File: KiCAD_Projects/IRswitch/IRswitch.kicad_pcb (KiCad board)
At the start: 2 copper layers, 39.4 x 45.7 mm, 14 parts, among them IC1 ATMEGA168-P, P1 CONN_01X02, P2 CONN_01X03, P3 CONN_01X05, Q1 MOSFET_N, X1 CRYSTAL

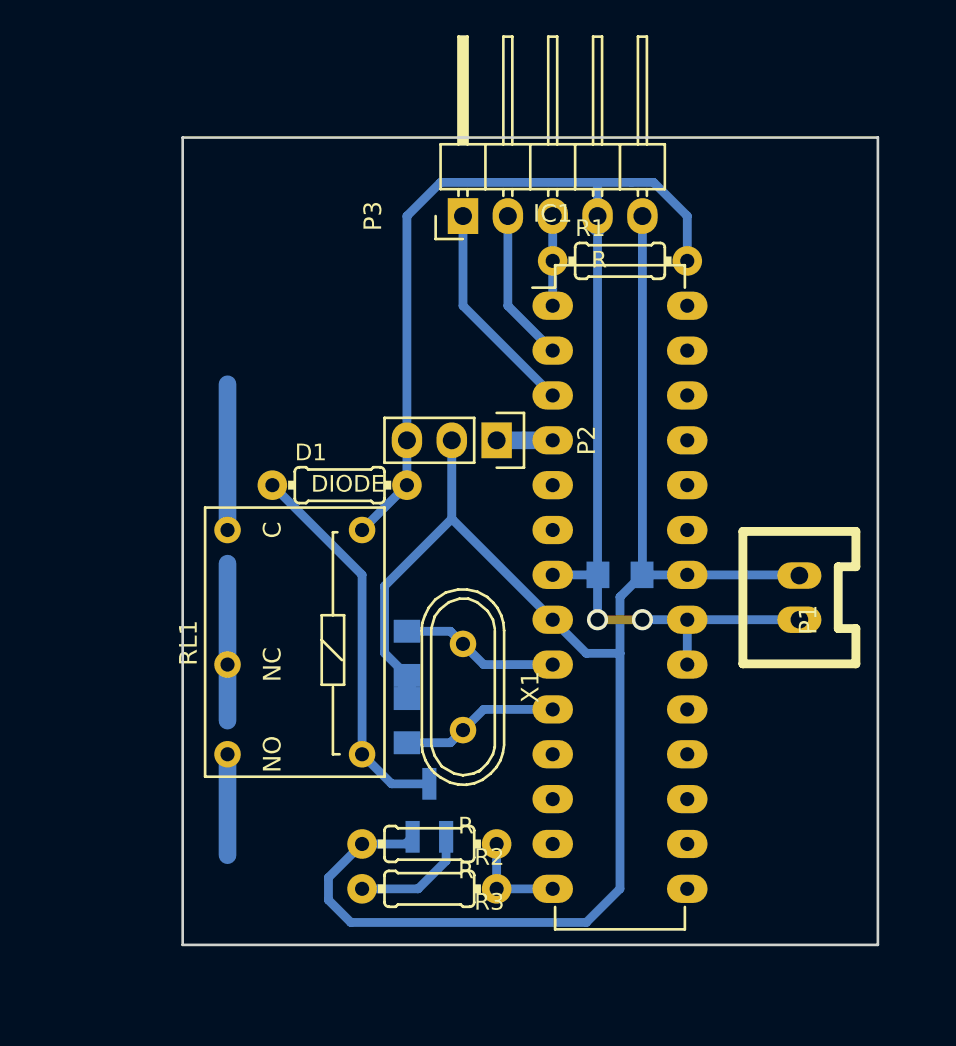
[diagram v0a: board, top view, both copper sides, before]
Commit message: no message
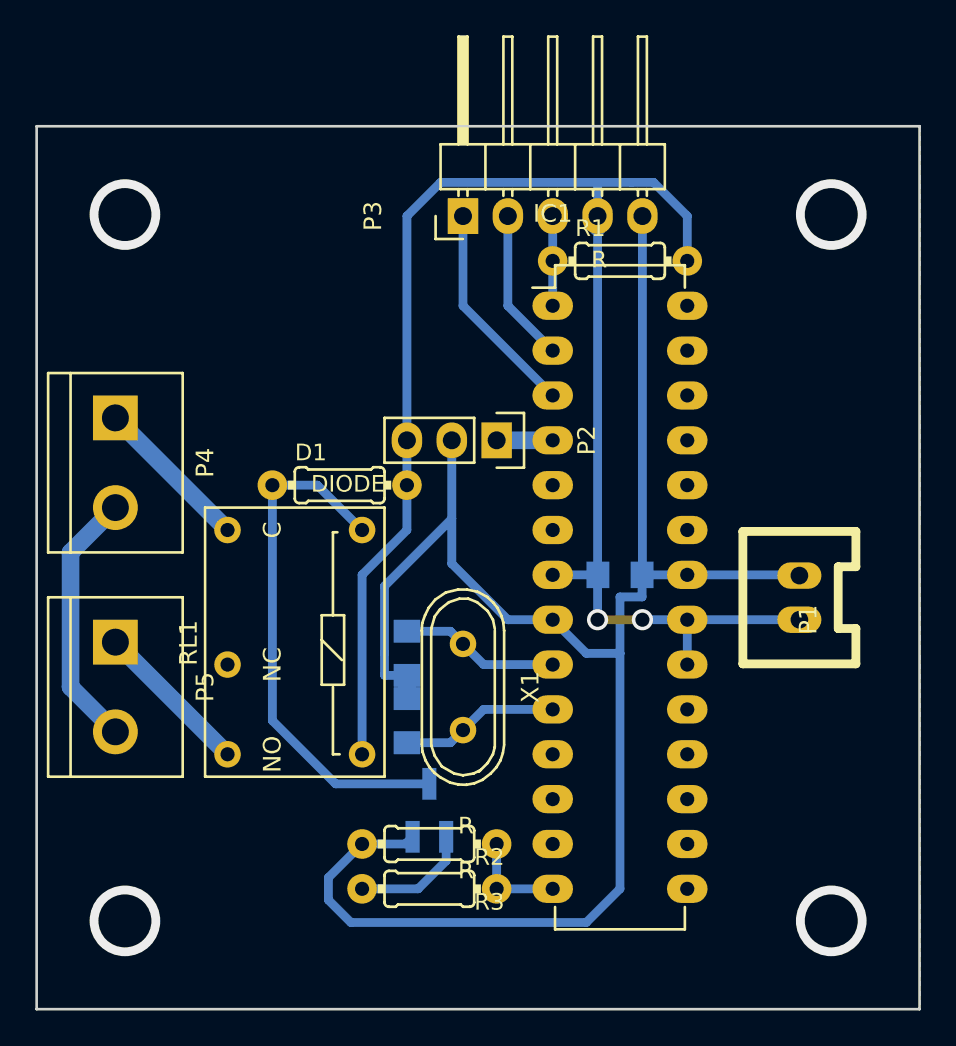
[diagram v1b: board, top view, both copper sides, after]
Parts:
- added P4: CONN_01X02, Connect:bornier2, F.Cu at (124.5, 59.1)
- added P5: CONN_01X02, Connect:bornier2, F.Cu at (124.5, 71.8)
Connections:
- IC1 pad 11: Net-(IC1-Pad11) -> (no net)
- IC1 pad 12: Net-(IC1-Pad12) -> (no net)
- IC1 pad 13: Net-(IC1-Pad13) -> (no net)
- IC1 pad 15: Net-(IC1-Pad15) -> (no net)
- IC1 pad 16: Net-(IC1-Pad16) -> (no net)
- IC1 pad 17: Net-(IC1-Pad17) -> (no net)
- IC1 pad 18: Net-(IC1-Pad18) -> (no net)
- IC1 pad 19: Net-(IC1-Pad19) -> (no net)
- IC1 pad 23: Net-(IC1-Pad23) -> (no net)
- IC1 pad 24: Net-(IC1-Pad24) -> (no net)
- IC1 pad 25: Net-(IC1-Pad25) -> (no net)
- IC1 pad 26: Net-(IC1-Pad26) -> (no net)
- IC1 pad 27: Net-(IC1-Pad27) -> (no net)
- IC1 pad 28: Net-(IC1-Pad28) -> (no net)
- IC1 pad 5: Net-(IC1-Pad5) -> (no net)
- IC1 pad 6: Net-(IC1-Pad6) -> (no net)
- RL1 pad 1: Net-(D1-Pad1) -> +5V
- RL1 pad 10: Net-(RL1-Pad10) -> (no net)
- RL1 pad 6: +5V -> Net-(D1-Pad1)
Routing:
- net Net-(P4-Pad2): track 0.00 -> 14.8 mm
- net +5V: track 80.8 -> 93.5 mm
- net Net-(RL1-Pad10): track 8.89 -> 0.00 mm
- net Net-(D1-Pad1): track 21.8 -> 29.8 mm
- net Net-(P5-Pad1): track 5.72 -> 8.98 mm
- net GND: track 101.8 -> 104.7 mm
- net Net-(P4-Pad1): track 8.26 -> 8.98 mm
- net (no net): vias 0 -> 4
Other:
- board size 39.4 x 45.7 mm -> 50 x 50 mm

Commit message: no message
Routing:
- added copper zone on B.Cu, net (none)
- removed copper zone on B.Cu, net GND
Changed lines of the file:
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@@
-(kicad_pcb (version 4) (host pcbnew 4.0.2-stable)
+(kicad_pcb (version 4) (host pcbnew 4.0.3-stable)
   (general
     (links 35)
     (no_connects 0)
-    (area 119.924999 39.924999 170.075001 90.075001)
+    (area 118.405 34.209999 170.075001 90.075001)
     (thickness 1.6)
     (drawings 4)
@@
   )
   (setup
-    (last_trace_width 0.5)
+    (last_trace_width 0.25)
     (user_trace_width 0.5)
     (user_trace_width 1)
@@
   (via (at 125 45) (size 4) (drill 3) (layers F.Cu B.Cu) (net 0))
   (via (at 165 45) (size 4) (drill 3) (layers F.Cu B.Cu) (net 0))
-  (segment (start 140.97 71.1) (end 139.72 71.1) (width 0.5) (layer B.Cu) (net 1) (status 400000))
+  (segment (start 140.97 71.1) (end 139.72 71.1) (width 0.5) (layer B.Cu) (net 1))
   (segment (start 139.7 71.08) (end 139.7 69.83) (width 0.5) (layer B.Cu) (net 1))
   (segment (start 139.72 71.1) (end 139.7 71.08) (width 0.5) (layer B.Cu) (net 1))
-  (segment (start 154.285 65.405) (end 154.285 66.655) (width 0.5) (layer B.Cu) (net 1) (status 400000))
+  (segment (start 154.285 65.405) (end 154.285 66.655) (width 0.5) (layer B.Cu) (net 1))
   (segment (start 154.285 66.655) (end 153.035 66.655) (width 0.5) (layer B.Cu) (net 1))
-  (segment (start 149.225 67.945) (end 146.685 67.945) (width 0.5) (layer B.Cu) (net 1) (status 400000))
+  (segment (start 149.225 67.945) (end 146.685 67.945) (width 0.5) (layer B.Cu) (net 1))
   (segment (start 143.51 64.77) (end 143.51 62.23) (width 0.5) (layer B.Cu) (net 1))
   (segment (start 146.685 67.945) (end 143.51 64.77) (width 0.5) (layer B.Cu) (net 1))
@@
   (segment (start 143.19 81.6) (end 141.605 83.185) (width 0.5) (layer B.Cu) (net 11))
   (segment (start 141.605 83.185) (end 138.43 83.185) (width 0.5) (layer B.Cu) (net 11))
-  (segment (start 124.46 56.515) (end 130.81 62.865) (width 1) (layer B.Cu) (net 12) (status C00000))
-  (segment (start 124.46 61.595) (end 121.92 64.135) (width 1) (layer B.Cu) (net 13) (status 400000))
-  (segment (start 121.92 71.755) (end 124.46 74.295) (width 1) (layer B.Cu) (net 13) (status 800000))
+  (segment (start 124.46 56.515) (end 130.81 62.865) (width 1) (layer B.Cu) (net 12))
+  (segment (start 124.46 61.595) (end 121.92 64.135) (width 1) (layer B.Cu) (net 13))
+  (segment (start 121.92 71.755) (end 124.46 74.295) (width 1) (layer B.Cu) (net 13))
   (segment (start 121.92 64.135) (end 121.92 71.755) (width 1) (layer B.Cu) (net 13))
   (segment (start 124.46 69.215) (end 130.81 75.565) (width 1) (layer B.Cu) (net 14))
-  (zone (net 1) (net_name GND) (layer B.Cu) (hatch edge 0.508)
+  (zone (net 0) (net_name "") (layer B.Cu) (hatch edge 0.508)
     (connect_pads (clearance 0.4))
     (min_thickness 0.2)
@@
     (polygon
       (pts
-        (xy 170 90) (xy 120 90) (xy 120 40) (xy 170 40) (xy 170 90)
+        (xy 170 90) (xy 120 90) (xy 120 40) (xy 170 40)
       )
     )
